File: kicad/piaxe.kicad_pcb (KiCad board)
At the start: 4 copper layers, 85 x 56 mm, 110 parts, among them J1 Barrel_Jack_Switch, J2 Conn_02x20_Odd_Even, J3 Conn_01x05, M1 Fan_4pin, Q1 CSD17576Q5B, Q2 CSD17308Q3, Q5 BSS138, Q6 BSS138, Q9 BSS138, U1 TPS40305, U13 TMP1075, U14 BM1366_mode1, U15 2N7001TDCK, U16 2N7001TDCK, U5 MCP1824T-1802E, U6 MCP1824T-0802E, U7 25MHz

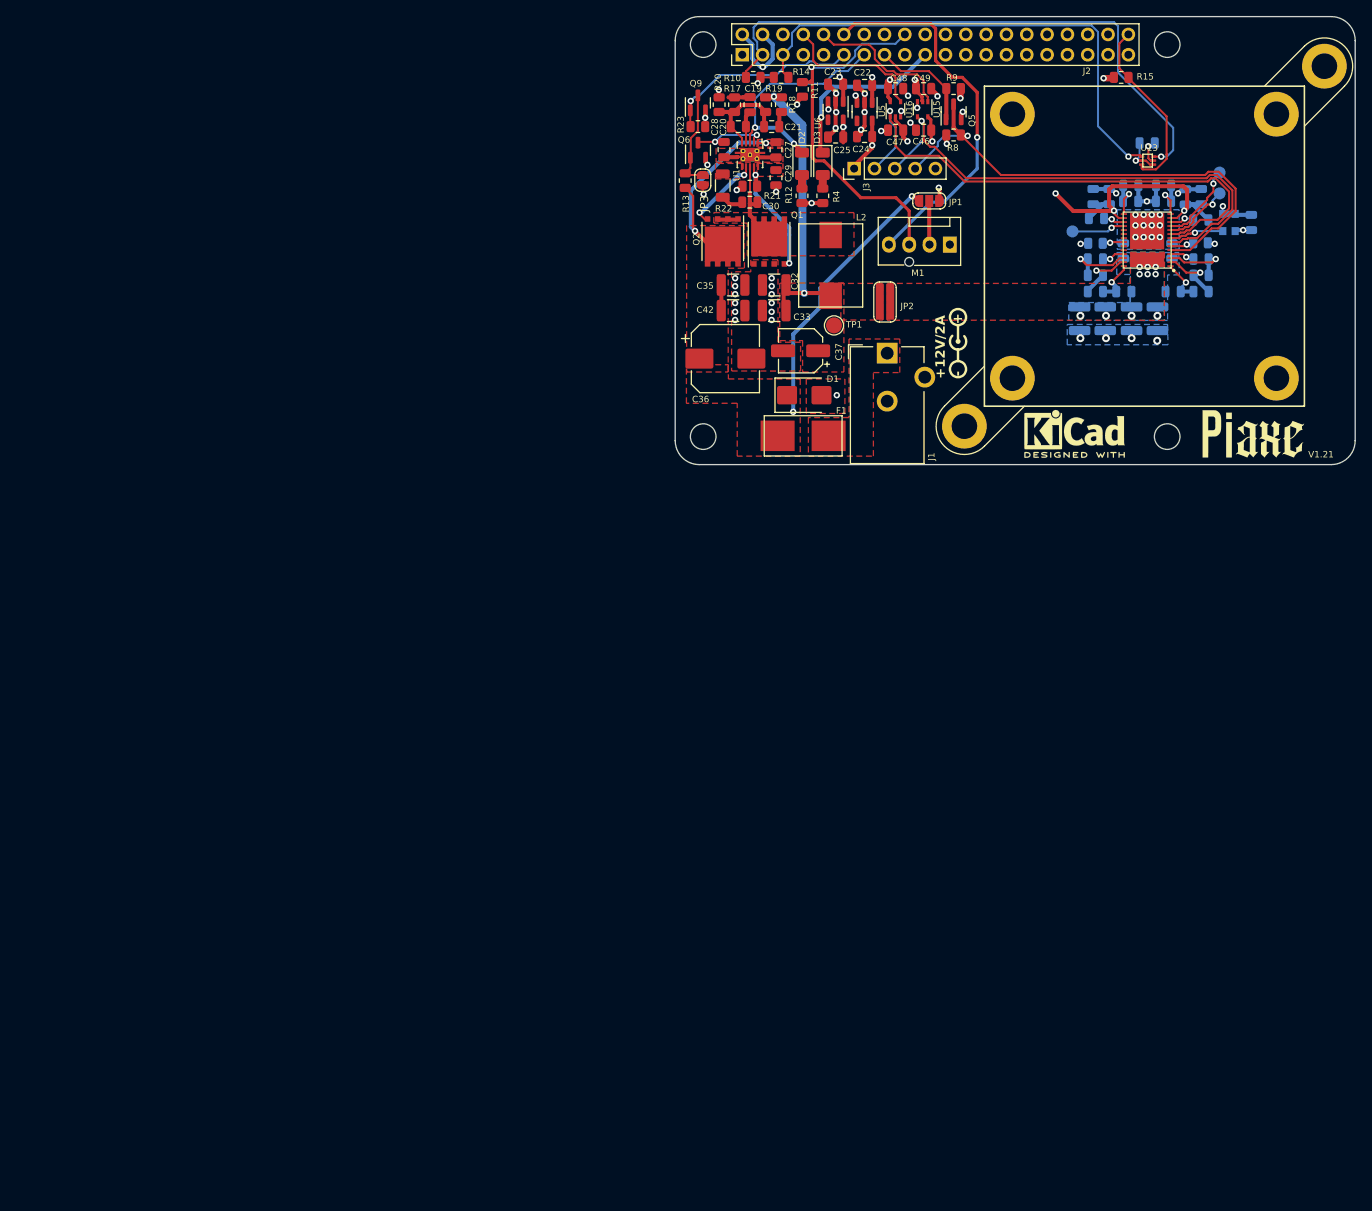
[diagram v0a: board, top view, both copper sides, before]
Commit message: initial commit before replacing power supply
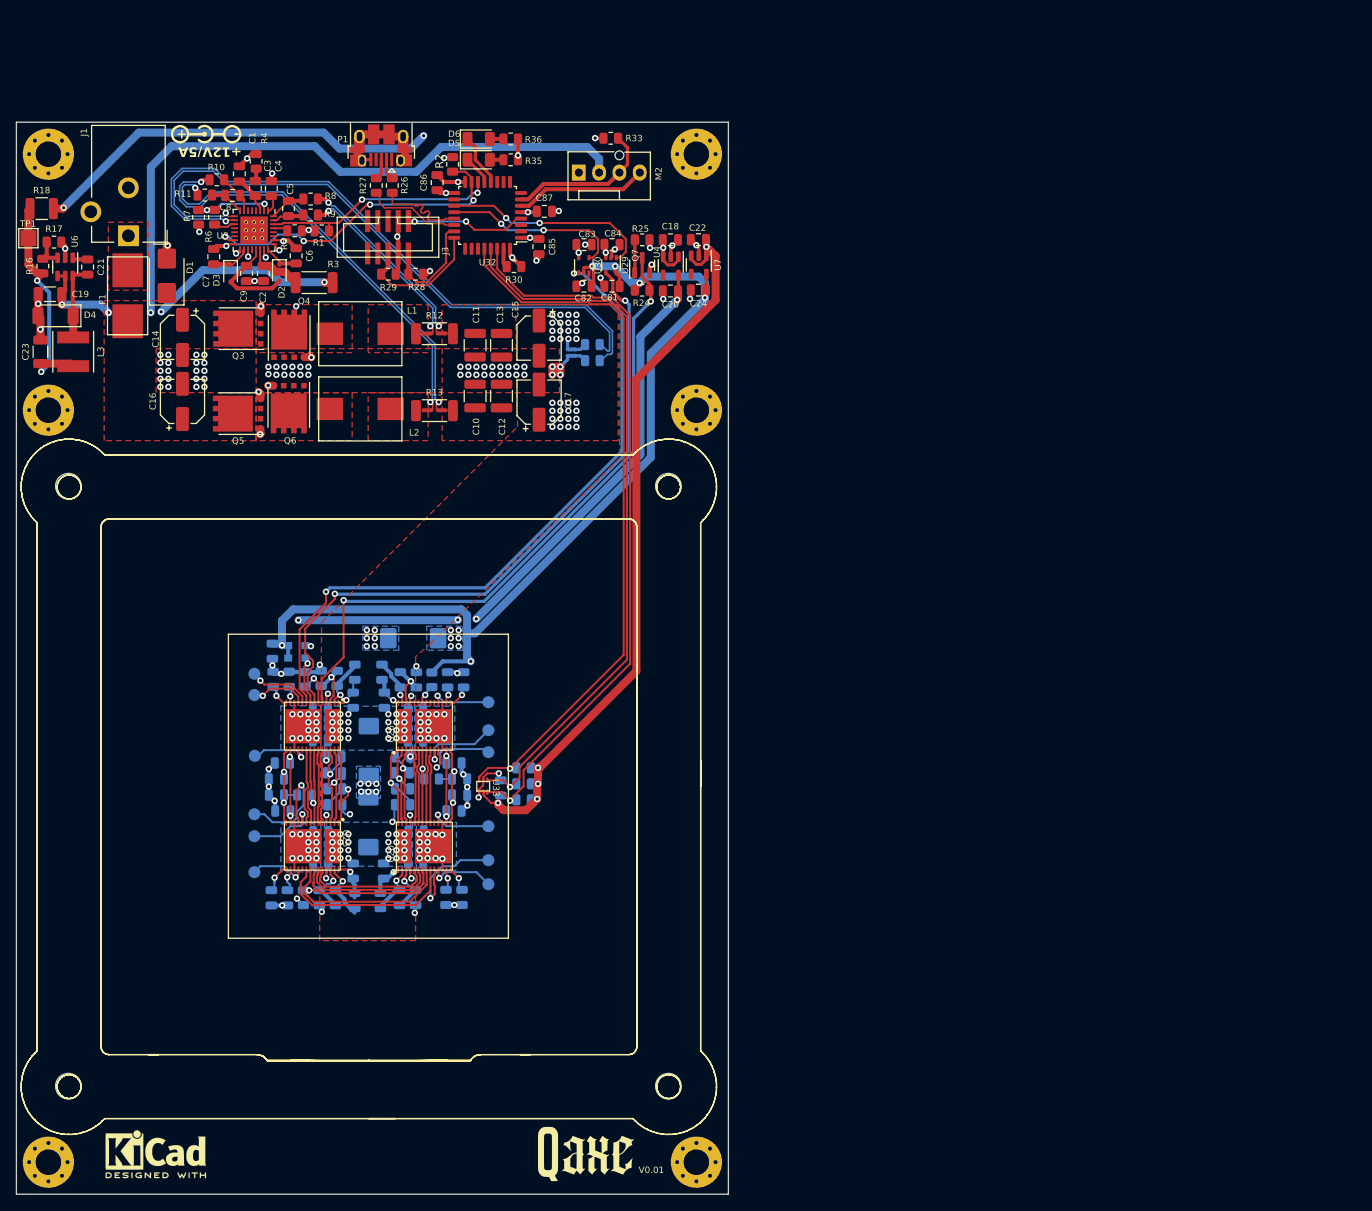
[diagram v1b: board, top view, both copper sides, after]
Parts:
- removed the C25 at (193.4, 70.9)
- removed the C35 at (180.6, 89.3)
- removed the C42 at (180.6, 92.5)
- removed the G*** at (248.9, 128.8)
- removed the G*** at (245.6, 108.0)
- removed H1, H2, H3, H4, H5, H6: MountingHole, MountingHole:MountingHole_3.2mm_M3_DIN965_Pad
- removed J2: Conn_02x20_Odd_Even, Connector_PinHeader_2.54mm:PinHeader_2x20_P2.54mm_Vertical
- removed JP1: SolderJumper_3_Open, Jumper:SolderJumper-3_P1.3mm_Open_RoundedPad1.0x1.5mm
- removed JP2: SolderJumper_2_Open, myfootprints:SolderJumper1.0x4.5
- removed JP3: SolderJumper_2_Open, Jumper:SolderJumper-2_P1.3mm_Open_RoundedPad1.0x1.5mm
- removed Q1: CSD17576Q5B, Package_SON:VSONP-8-1EP_5x6_P1.27mm
- removed Q2: CSD17308Q3, Package_SON:VSONP-8-1EP_5x6_P1.27mm
- removed Q9: BSS138, Package_TO_SOT_SMD:SOT-23
- removed the R1 at (225.9, 84.1)
- removed the R19 at (184.6, 66.8)
- removed the REF** at (176.8, 108.3)
- removed the REF** at (234.8, 108.3)
- removed the REF** at (176.8, 59.3)
- removed the REF** at (234.8, 59.3)
- removed the U1 at (182.7, 73.1)
- removed U14: BM1366_mode1, bitaxe:BM1366
- removed U5: MCP1824T-1802E, Package_TO_SOT_SMD:SOT-23-5
- added C1: 47p, Capacitor_SMD:C_0805_2012Metric, F.Cu at (118.9, 75.5)
- added C12: 100µ/6.3V, Capacitor_SMD:C_1210_3225Metric, F.Cu at (151.6, 103.2)
- added C14: 220µ, Capacitor_SMD:CP_Elec_5x5.8, F.Cu at (111.8, 95.9)
- added C15: 330µ, Capacitor_SMD:CP_Elec_5x5.8, F.Cu at (156.3, 96.0)
- added C16: 220µ, Capacitor_SMD:CP_Elec_5x5.8, F.Cu at (111.8, 103.9)
- added C17: 330µ, Capacitor_SMD:CP_Elec_5x5.8, F.Cu at (156.3, 104.0)
- added C18: 100n, Capacitor_SMD:C_0805_2012Metric, F.Cu at (172.8, 83.7)
- added C2: 100n, Capacitor_SMD:C_0805_2012Metric, F.Cu at (121.9, 87.9)
- added C26: 10µ, Capacitor_SMD:C_0805_2012Metric, B.Cu at (129.0, 146.3)
- added C3: 3.3n, Capacitor_SMD:C_0805_2012Metric, F.Cu at (120.9, 77.3)
- added C44: 1µ, Capacitor_SMD:C_0805_2012Metric, B.Cu at (145.7, 155.1)
- added C45: 330µ/6.3V, Capacitor_Tantalum_SMD:CP_EIA-7343-15_Kemet-W, B.Cu at (135.0, 156.5)
- added C46: 1µ, Capacitor_SMD:C_0805_2012Metric, B.Cu at (140.9, 157.6)
- added C47: 1µ, Capacitor_SMD:C_0805_2012Metric, B.Cu at (124.3, 155.1)
- added C48: 330µ/6.3V, Capacitor_Tantalum_SMD:CP_EIA-7343-15_Kemet-W, B.Cu at (135.1, 147.6)
- added C49: 100n, Capacitor_SMD:C_0805_2012Metric, B.Cu at (129.1, 144.3)
- added C51: 1µ, Capacitor_SMD:C_0805_2012Metric, B.Cu at (136.5, 166.3)
- added C53: 100n, Capacitor_SMD:C_0805_2012Metric, B.Cu at (129.1, 159.7)
- added C55: 100n, Capacitor_SMD:C_0805_2012Metric, B.Cu at (140.9, 159.6)
- added C57: 1µ, Capacitor_SMD:C_0805_2012Metric, B.Cu at (136.9, 162.6)
- added C59: 100n, Capacitor_SMD:C_0805_2012Metric, B.Cu at (140.9, 144.3)
- added C6: 100n, Capacitor_SMD:C_0805_2012Metric, F.Cu at (126.0, 85.7)
- added C61: 1µ, Capacitor_SMD:C_0805_2012Metric, B.Cu at (146.4, 151.1)
- added C63: 1µ, Capacitor_SMD:C_0805_2012Metric, B.Cu at (139.3, 154.3)
- added C64: 1µ, Capacitor_SMD:C_0805_2012Metric, B.Cu at (146.4, 153.1)
- added C65: 1µ, Capacitor_SMD:C_0805_2012Metric, B.Cu at (123.5, 153.1)
- added C67: 1µ, Capacitor_SMD:C_0805_2012Metric, B.Cu at (139.3, 152.3)
- added C68: 1µ, Capacitor_SMD:C_0805_2012Metric, B.Cu at (123.5, 151.1)
- added C70: 1µ, Capacitor_SMD:C_0805_2012Metric, B.Cu at (139.2, 150.3)
- added C72: 1µ, Capacitor_SMD:C_0805_2012Metric, B.Cu at (139.3, 148.3)
- added C73: 1µ, Capacitor_SMD:C_0805_2012Metric, B.Cu at (133.1, 162.6)
- added C74: 1µ, Capacitor_SMD:C_0805_2012Metric, B.Cu at (137.0, 141.2)
- added C75: 1µ, Capacitor_SMD:C_0805_2012Metric, B.Cu at (133.3, 166.3)
- added C76: 1µ, Capacitor_SMD:C_0805_2012Metric, B.Cu at (136.7, 137.8)
- added C77: 1µ, Capacitor_SMD:C_0805_2012Metric, B.Cu at (130.9, 165.9)
- added C78: 1µ, Capacitor_SMD:C_0805_2012Metric, B.Cu at (139.0, 138.7)
- added C79: 1µ, Capacitor_SMD:C_0805_2012Metric, B.Cu at (128.9, 165.9)
- added C8: 1n, Capacitor_SMD:C_0805_2012Metric, F.Cu at (118.0, 78.2)
- added C80: 1µ, Capacitor_SMD:C_0805_2012Metric, B.Cu at (141.0, 138.7)
- added C85: 100n, Capacitor_SMD:C_0805_2012Metric, F.Cu at (156.3, 84.5)
- added C86: 100n, Capacitor_SMD:C_0805_2012Metric, F.Cu at (143.6, 76.5)
- added C87: 100n, Capacitor_SMD:C_0805_2012Metric, F.Cu at (157.0, 80.2)
- added D2: D_Schottky_Small, Diode_SMD:D_SOD-323, F.Cu at (123.9, 87.8)
- added D3: D_Schottky_Small, Diode_SMD:D_SOD-323, F.Cu at (117.8, 87.9)
- added D4: PMEG4030EP,115, Diode_SMD:D_SOD-128, F.Cu at (95.9, 93.2)
- added G***: LOGO, bitaxe:qaxelogo, F.Cu at (162.2, 198.0)
- added L1: 220nH, myfootprints:IFLR-4031GC-01-8x10, F.Cu at (134.0, 95.4)
- added L3: 4.7µH/2A/3A, Inductor_SMD:L_Taiyo-Yuden_NR-50xx, F.Cu at (98.1, 97.7)
- added NT1: NetTie_2, NetTie:NetTie-2_SMD_Pad0.5mm, F.Cu at (142.4, 95.4)
- added NT2: NetTie_2, NetTie:NetTie-2_SMD_Pad0.5mm, F.Cu at (142.4, 105.0)
- added NT3: NetTie_2, NetTie:NetTie-2_SMD_Pad0.5mm, F.Cu at (144.2, 95.4)
- added NT4: NetTie_2, NetTie:NetTie-2_SMD_Pad0.5mm, F.Cu at (144.2, 105.0)
- added NT5: NetTie_2, NetTie:NetTie-2_SMD_Pad0.5mm, B.Cu at (160.4, 97.4)
- added NT6: NetTie_2, NetTie:NetTie-2_SMD_Pad0.5mm, B.Cu at (160.4, 98.2)
- added P1: MYUSB_B, Connector_USB:USB_Micro-B_Amphenol_10103594-0001LF_Horizontal, F.Cu at (136.6, 71.9)
- added Q3: CSD17308Q3, Package_SON:VSONP-8-1EP_5x6_P1.27mm, F.Cu at (118.7, 94.8)
- added Q4: CSD17308Q3, Package_SON:VSONP-8-1EP_5x6_P1.27mm, F.Cu at (125.1, 95.6)
- added Q5: CSD17308Q3, Package_SON:VSONP-8-1EP_5x6_P1.27mm, F.Cu at (118.7, 105.4)
- added R12: 0.001, Resistor_SMD:R_2010_5025Metric, F.Cu at (143.3, 95.4)
- added R16: 49,9k, Resistor_SMD:R_0805_2012Metric, F.Cu at (94.3, 87.0)
- added R2: 1.5k, Resistor_SMD:R_0805_2012Metric, F.Cu at (145.5, 74.3)
- added R23: 10k, Resistor_SMD:R_0805_2012Metric, B.Cu at (126.9, 165.9)
- added R26: 22, Resistor_SMD:R_0805_2012Metric, F.Cu at (138.0, 76.9)
- added R27: 22, Resistor_SMD:R_0805_2012Metric, F.Cu at (136.0, 76.9)
- added R28: 10k, Resistor_SMD:R_0805_2012Metric, F.Cu at (140.9, 88.0)
- added R29: 10k, Resistor_SMD:R_0805_2012Metric, F.Cu at (137.5, 88.0)
- added R3: 2.2R, Resistor_SMD:R_2010_5025Metric, F.Cu at (128.2, 89.1)
- added R30: 100k, Resistor_SMD:R_0805_2012Metric, F.Cu at (153.2, 87.0)
- added R31: 10k, Resistor_SMD:R_0805_2012Metric, B.Cu at (154.4, 149.7)
- added R32: 1.5k, Resistor_SMD:R_0805_2012Metric, B.Cu at (154.4, 151.7)
- added R33: 2k2, Resistor_SMD:R_0805_2012Metric, F.Cu at (165.3, 71.0)
- added R34: 1.5k, Resistor_SMD:R_0805_2012Metric, B.Cu at (154.4, 153.7)
- added R4: 8.45k, Resistor_SMD:R_0805_2012Metric, F.Cu at (121.0, 73.9)
- added R5: 100k, Resistor_SMD:R_0805_2012Metric, F.Cu at (125.8, 82.6)
- added R6: 20k, Resistor_SMD:R_0805_2012Metric, F.Cu at (115.8, 80.9)
- added R7: 20k, Resistor_SMD:R_0805_2012Metric, F.Cu at (113.8, 80.9)
- added R8: 200, Resistor_SMD:R_0805_2012Metric, F.Cu at (127.8, 78.6)
- added R9: 200, Resistor_SMD:R_0805_2012Metric, F.Cu at (127.8, 80.6)
- added REF**: MountingHole_3.2mm_M3_Pad_Via, MountingHole:MountingHole_3.2mm_M3_Pad_Via, F.Cu at (95.0, 73.0)
- added REF**: MountingHole_3.2mm_M3_Pad_Via, MountingHole:MountingHole_3.2mm_M3_Pad_Via, F.Cu at (95.0, 199.0)
- added REF**: MountingHole_3.2mm_M3, MountingHole:MountingHole_3.2mm_M3, F.Cu at (172.5, 189.5)
- added REF**: MountingHole_3.2mm_M3, MountingHole:MountingHole_3.2mm_M3, F.Cu at (97.5, 189.5)
- added REF**: MountingHole_3.2mm_M3, MountingHole:MountingHole_3.2mm_M3, F.Cu at (97.5, 114.5)
- added REF**: MountingHole_3.2mm_M3_Pad_Via, MountingHole:MountingHole_3.2mm_M3_Pad_Via, F.Cu at (176.0, 73.0)
- added REF**: MountingHole_3.2mm_M3, MountingHole:MountingHole_3.2mm_M3, F.Cu at (172.5, 114.5)
- added REF**: MountingHole_3.2mm_M3_Pad_Via, MountingHole:MountingHole_3.2mm_M3_Pad_Via, F.Cu at (176.0, 199.0)
- added REF**: MountingHole_3.2mm_M3_Pad_Via, MountingHole:MountingHole_3.2mm_M3_Pad_Via, F.Cu at (95.0, 105.0)
- added REF**: MountingHole_3.2mm_M3_Pad_Via, MountingHole:MountingHole_3.2mm_M3_Pad_Via, F.Cu at (176.0, 105.0)
- added TP10: TestPoint, TestPoint:TestPoint_Pad_D1.5mm, B.Cu at (150.0, 145.0)
- added TP11: TestPoint, TestPoint:TestPoint_Pad_D1.5mm, B.Cu at (150.0, 147.8)
- added TP12: TestPoint, TestPoint:TestPoint_Pad_D1.5mm, B.Cu at (150.0, 141.5)
- added TP13: TestPoint, TestPoint:TestPoint_Pad_D1.5mm, B.Cu at (120.8, 162.8)
- added TP4: TestPoint, TestPoint:TestPoint_Pad_D1.5mm, B.Cu at (150.0, 161.2)
- added TP5: TestPoint, TestPoint:TestPoint_Pad_D1.5mm, B.Cu at (150.0, 164.2)
- added TP7: TestPoint, TestPoint:TestPoint_Pad_D1.5mm, B.Cu at (150.0, 157.0)
- added TP8: TestPoint, TestPoint:TestPoint_Pad_D1.5mm, B.Cu at (120.8, 158.2)
- added TP9: TestPoint, TestPoint:TestPoint_Pad_D1.5mm, B.Cu at (120.8, 155.5)
- added U19: BM1366_mode1, bitaxe:BM1366, F.Cu at (128.0, 144.5)
- added U20: BM1366_mode1, bitaxe:BM1366, F.Cu at (142.0, 159.5)
- added U25: BM1366_mode1, bitaxe:BM1366, F.Cu at (128.0, 159.5)
- added U26: BM1366_mode1, bitaxe:BM1366, F.Cu at (142.0, 144.5)
- added U3: LTC3856, Package_DFN_QFN:QFN-32-1EP_5x5mm_P0.5mm_EP3.45x3.45mm_ThermalVias, F.Cu at (120.7, 82.5)
- added U32: STM32L052K6Tx, Package_QFP:LQFP-32_7x7mm_P0.8mm, F.Cu at (149.9, 80.7)
- added U4: MCP1824T-0802E, Package_TO_SOT_SMD:SOT-23-5, F.Cu at (172.8, 87.0)
- added U7: MCP1824T-1802E, Package_TO_SOT_SMD:SOT-23-5, F.Cu at (176.3, 86.8)
- C10, C11: value 1µ -> 100µ/6.3V; footprint Capacitor_SMD:C_0805_2012Metric -> Capacitor_SMD:C_1210_3225Metric; moved to F.Cu
- C13: value 100n -> 100µ/6.3V; footprint Capacitor_SMD:C_0805_2012Metric -> Capacitor_SMD:C_1210_3225Metric; moved to F.Cu
- C19: value 1.5n -> 10µF/50V; footprint Capacitor_SMD:C_0805_2012Metric -> Capacitor_SMD:C_1206_3216Metric
- C20: value 180p -> 1µ
- C21: value 560p -> 10n/250V
- C23: value 100n -> 22µ/16V; footprint Capacitor_SMD:C_0805_2012Metric -> Capacitor_SMD:C_1206_3216Metric
- C27: value 1µ -> 10µ; moved to B.Cu
- C28: value 3.3n -> 1µ; moved to B.Cu
- C29: value 4.7µ/25V -> 10µ; moved to B.Cu
- C30: value 100n -> 1µ; moved to B.Cu
- C31: value 1µ -> 10µ
- C32, C33: value 47µ/6.3V -> 1µ; footprint Capacitor_SMD:C_1210_3225Metric -> Capacitor_SMD:C_0805_2012Metric; moved to B.Cu
- C36: value 330µ -> 1µ; footprint Capacitor_SMD:CP_Elec_8x10 -> Capacitor_SMD:C_0805_2012Metric; moved to B.Cu
- C37: value 220µ -> 1µ; footprint Capacitor_SMD:CP_Elec_5x5.8 -> Capacitor_SMD:C_0805_2012Metric; moved to B.Cu
- C38: value 10µ/25V -> 1µ; footprint Capacitor_SMD:C_1210_3225Metric -> Capacitor_SMD:C_0805_2012Metric
- C39: value 10µ/25V -> 330µ/6.3V; footprint Capacitor_SMD:C_1210_3225Metric -> Capacitor_Tantalum_SMD:CP_EIA-7343-15_Kemet-W
- C4: value 1µ -> 100n; moved to F.Cu
- C40, C41: value 47µ/6.3V -> 1µ; footprint Capacitor_SMD:C_1210_3225Metric -> Capacitor_SMD:C_0805_2012Metric
- C43: value 100n -> 1µ
- C5: value 1µ -> 1n; moved to F.Cu
- C58: renamed from C44; value 100n -> 1µ
- C60: renamed from C45; value 100n -> 1µ
- C7: moved to F.Cu
- C9: value 100n -> 4.7µ; moved to F.Cu
- J3: value Conn_01x05 -> SWD; footprint Connector_PinHeader_2.54mm:PinHeader_1x05_P2.54mm_Vertical -> myfootprints:PinHeader_IDC_2x05_P1.27mm_Vertical_SMD
- L2: value 170nH -> 220nH
- Q6: value BSS138 -> CSD17308Q3; footprint Package_TO_SOT_SMD:SOT-23 -> Package_SON:VSONP-8-1EP_5x6_P1.27mm
- R10: value 1.5k -> 200
- R11: value 2k2 -> 200
- R13: value 10k -> 0.001; footprint Resistor_SMD:R_0805_2012Metric -> Resistor_SMD:R_2010_5025Metric
- R14: value 1.5k -> 10; moved to B.Cu
- R15: value 10k -> 10; moved to B.Cu
- R17: value 4.3k -> 16.3k
- R18: value 1.24k -> 0; footprint Resistor_SMD:R_0805_2012Metric -> Resistor_SMD:R_1210_3225Metric
- R20, R21: moved to B.Cu
- R22: value 0 -> 10k; footprint Resistor_SMD:R_1206_3216Metric -> Resistor_SMD:R_0805_2012Metric; moved to B.Cu
- TP1: value +1V2 -> 3V3; footprint TestPoint:TestPoint_Pad_D2.0mm -> TestPoint:TestPoint_Pad_2.0x2.0mm
- U6: value MCP1824T-0802E -> AP3211; footprint Package_TO_SOT_SMD:SOT-23-5 -> Package_TO_SOT_SMD:SOT-23-6
- moved REF** 145.9 mm to (108.4, 198.0)
- moved C52 141.5 mm to (122.9, 165.9), turned to -90 degrees
- moved TP3 137.2 mm to (120.8, 140.6)
- moved TP2 134.8 mm to (120.8, 137.9)
- moved C25 133.6 mm to (123.0, 135.1)
- moved C43 133.1 mm to (138.9, 165.9)
- moved U8 128.3 mm to (126.0, 135.2), turned to -90 degrees
- moved C31 126.9 mm to (140.9, 161.6), turned to 0 degrees
- moved R19 124.5 mm to (127.1, 138.6), turned to -90 degrees
- moved C60 123.7 mm to (123.1, 138.6), turned to 90 degrees
- moved C38 122.7 mm to (129.1, 157.7), turned to 180 degrees
- moved C35 121.8 mm to (129.1, 138.5), turned to -90 degrees
- moved TP6 121.4 mm to (120.8, 148.2)
- moved C54 120.6 mm to (146.7, 165.9), turned to -90 degrees
- moved C42 119.2 mm to (131.1, 138.5), turned to -90 degrees
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- renumbered C1 to C25, C2 to C35, C3 to C42, C6 to C50, C16 to C52, C14 to C54, C8 to C56, C12 to C62, C15 to C66, C17 to C69, C18 to C71, C46 to C81, C47 to C82, C48 to C83, C49 to C84, C26 to C88, D2 to D5, D3 to D6, M1 to M2, Q5 to Q7, R23 to R1, R6 to R19, R8 to R24, R9 to R25, R12 to R35, R4 to R36, TP3 to TP2, TP4 to TP3, TP2 to TP6, U3 to U1, U15 to U29, U16 to U30, U13 to U33, U7 to U8
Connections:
- C13 pad 1: +0V8 -> +1V2
- C19 pad 1: Net-(U1-COMP) -> +12V
- C19 pad 2: Net-(C19-Pad2) -> GND
- C20 pad 1: Net-(U1-COMP) -> +0V8
- C20 pad 2: Net-(U1-FB) -> GND
- C21 pad 1: Net-(C21-Pad1) -> Net-(U6-BS)
- C21 pad 2: Net-(U1-FB) -> Net-(D4-K)
- C22 pad 1: +5V -> +3V3
- C23 pad 1: +5V -> Net-(C23-Pad1)
- C27 pad 1: +12V -> +1V2
- C28 pad 1: Net-(Q6-D) -> GND
- C28 pad 2: GND -> +0V8
- C29 pad 1: Net-(U1-BP) -> +1V2
- C30 pad 1: Net-(C30-Pad1) -> GND
- C30 pad 2: Net-(Q1-D) -> +0V8
- C31 pad 1: +0V8 -> +1V2
- C32 pad 1: Net-(JP2-A) -> GND
- C32 pad 2: GND -> +0V8
- C33 pad 1: Net-(JP2-A) -> +1V2
- C36 pad 1: +12V -> GND
- C36 pad 2: GND -> Net-(U20-VDD3_0)
- C37 pad 1: Net-(JP2-A) -> GND
- C37 pad 2: GND -> +0V8
- C4 pad 1: +0V8 -> Net-(U3-TK/SS)
- C40 pad 1: +1V2 -> GND
- C40 pad 2: GND -> +0V8
- C43 pad 1: +0V8 -> Net-(U20-VDD3_0)
- C43 pad 2: GND -> Net-(U20-VDD2_0)
- C5 pad 1: +0V8 -> Net-(U3-SENSE1-)
- C5 pad 2: GND -> Net-(U3-SENSE1+)
- C7 pad 1: +1V2 -> Net-(D3-K)
- C7 pad 2: GND -> Net-(Q5-S)
- C9 pad 1: +1V2 -> Net-(D2-A)
- D5 pad 1: /Pi/PGOOD -> LED2
- D6 pad 1: Net-(D3-K) -> LED1
- J3 pad 1: +1V8 -> ARM_NRST
- J3 pad 2: /BM1366/CI -> ARM_SWDIO
- J3 pad 3: /BM1366/RO -> GND
- J3 pad 4: /BM1366/RST_N -> GND
- J3 pad 5: GND -> unconnected-(J3-Pin_5-Pad5)
- L2 pad 1: Net-(Q1-D) -> Net-(Q5-S)
- L2 pad 2: Net-(JP2-A) -> Net-(L2-Pad2)
- M2 pad 2: Net-(JP1-C) -> +12V
- M2 pad 3: /Pi/TACHO -> FAN_TACHO
- M2 pad 4: /Pi/PWM -> FAN_PWM
- Q6 pad 1: Net-(JP3-A) -> GND
- Q6 pad 2: GND -> Net-(Q6-G)
- Q6 pad 3: Net-(Q6-D) -> Net-(Q5-S)
- R1 pad 2: /Pi/SDN -> 1V2_RUN
- R10 pad 1: +3V3 -> Net-(U3-SENSE2+)
- R10 pad 2: /Pi/SDA -> /Power/SENSE2+
- R11 pad 1: +3V3 -> Net-(U3-SENSE2-)
- R11 pad 2: /Pi/TACHO -> /Power/SENSE2-
- R13 pad 1: Net-(JP3-A) -> Net-(L2-Pad2)
- R13 pad 2: +12V -> +1V2
- R14 pad 1: +3V3 -> Net-(NT5-Pad1)
- R14 pad 2: /Pi/SCL -> /Power/DIFF+
- R15 pad 1: +3V3 -> Net-(NT6-Pad1)
- R15 pad 2: /Pi/ALERT -> /Power/DIFF-
- R17 pad 1: Net-(C19-Pad2) -> Net-(U6-FB)
- R17 pad 2: Net-(U1-FB) -> GND
- R18 pad 1: Net-(JP2-A) -> Net-(C23-Pad1)
- R18 pad 2: Net-(C21-Pad1) -> +3V3
- R20 pad 1: GND -> Net-(U19-RI)
- R20 pad 2: Net-(U1-FB) -> +1V8
- R21 pad 2: GND -> +1V8
- R22 pad 2: Net-(C30-Pad1) -> +1V8
- TP1 pad 1: Net-(JP2-A) -> Net-(C23-Pad1)
- TP2 pad 1: /BM1366/TEMP_P -> Net-(U19-ADDR0)
- TP3 pad 1: /BM1366/TEMP_N -> Net-(U19-ADDR1)
- U29 pad 1: /Pi/RXD -> RX
- U30 pad 4: /Pi/TXD -> TX
- U33 pad 1: /Pi/SCL -> TMP_SCL
- U33 pad 3: /Pi/ALERT -> TMP_ALARM
- U33 pad 6: /Pi/SDA -> TMP_SDA
- U6 pad 1: +5V -> Net-(U6-BS)
- U6 pad 3: +5V -> Net-(U6-FB)
- U6 pad 4: unconnected-(U6-PG-Pad4) -> +12V
- U6 pad 5: +0V8 -> +12V
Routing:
- net +1V8: track 97.4 -> 230.5 mm, vias 8 -> 15
- net +0V8: track 74.9 -> 176.8 mm, vias 4 -> 12
- net TMP_SDA: track 0.00 -> 92.5 mm, vias 0 -> 1
- net TMP_SCL: track 0.00 -> 90.8 mm, vias 0 -> 1
- net TMP_ALARM: track 0.00 -> 90.0 mm, vias 0 -> 1
- net /Power/DIFF-: track 0.00 -> 81.1 mm, vias 0 -> 1
- net /Power/DIFF+: track 0.00 -> 78.5 mm, vias 0 -> 1
- net /Pi/SDA: track 74.8 -> 0.00 mm, vias 1 -> 0
- net GND: track 115.9 -> 189.9 mm, vias 58 -> 163
- net +5V: track 69.8 -> 0.00 mm, vias 6 -> 0
- net /Pi/SCL: track 64.3 -> 0.00 mm, vias 1 -> 0
- net +3V3: track 107.2 -> 170.8 mm, vias 8 -> 18
- net /Power/SENSE2+: track 0.00 -> 54.6 mm, vias 0 -> 2
- net /Power/SENSE2-: track 0.00 -> 53.6 mm, vias 0 -> 2
- net +12V: track 67.5 -> 115.4 mm, vias 4 -> 5
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- added copper zone on In1.Cu, net +1V2
- added copper zone on In1.Cu, net +3V3
- added copper zone on F.Cu, net Net-(L1-Pad2)
- added copper zone on F.Cu, net Net-(L2-Pad2)
- added copper zone on F.Cu, net Net-(Q3-S)
- added copper zone on F.Cu, net Net-(Q5-S)
- removed copper zone on F.Cu, net Net-(JP2-A)
- removed copper zone on F.Cu, net Net-(Q1-D)
- removed copper zone on F.Cu, net Net-(U1-BP)
- removed copper zone on F.Cu, net Net-(U26-RI)
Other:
- board size 85 x 56 mm -> 89 x 134 mm
- board text added: "+12V/5A"
- board text added: "V0.01"
- board text removed: "+12V/2A"
- board text removed: "V1.21"
